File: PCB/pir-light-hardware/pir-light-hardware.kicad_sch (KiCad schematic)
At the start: 38 parts, among them J1 ZH1.5-3, J2 ZH1.5-3, Q1 AON7240, Q2 NPN, Q3 PNP, U1 M74VHC1GT08DFT2G, U2 LMV331IDCKR, U3 AS312

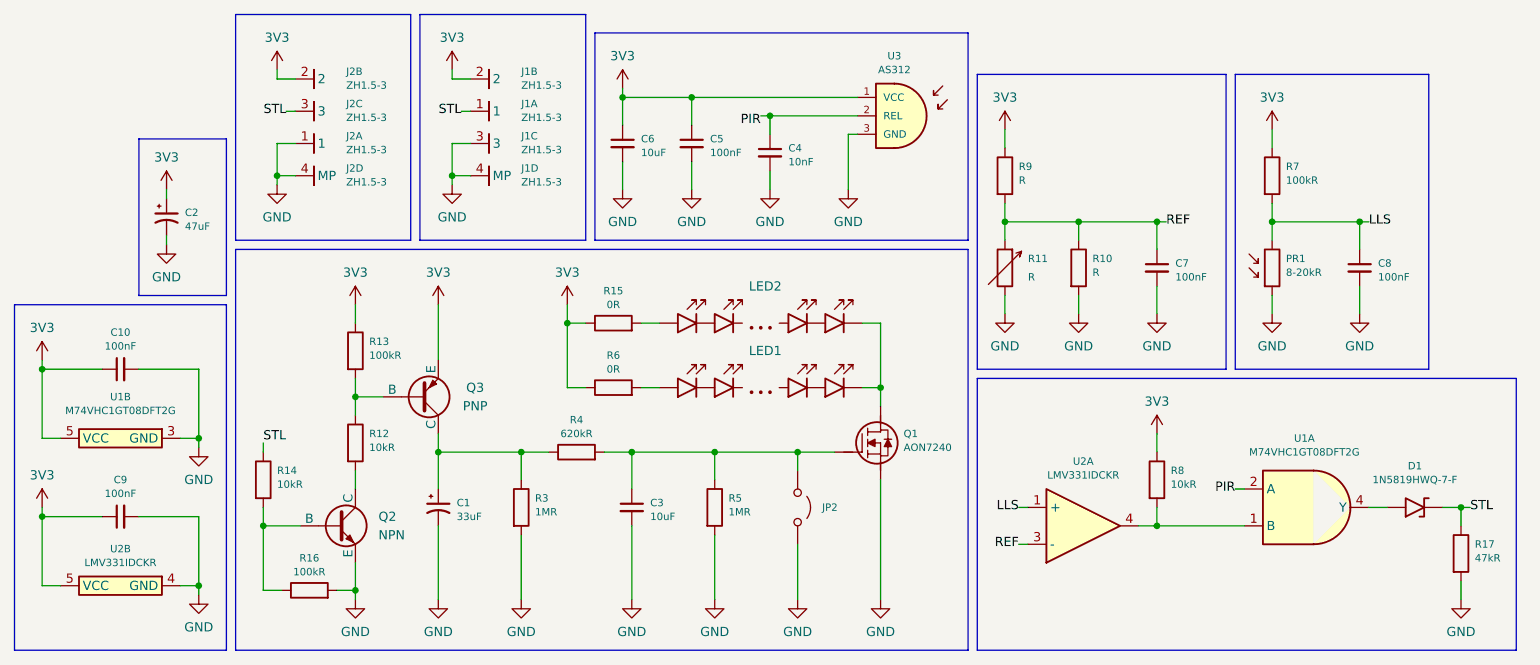
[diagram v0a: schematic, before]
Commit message: chore: add protection components
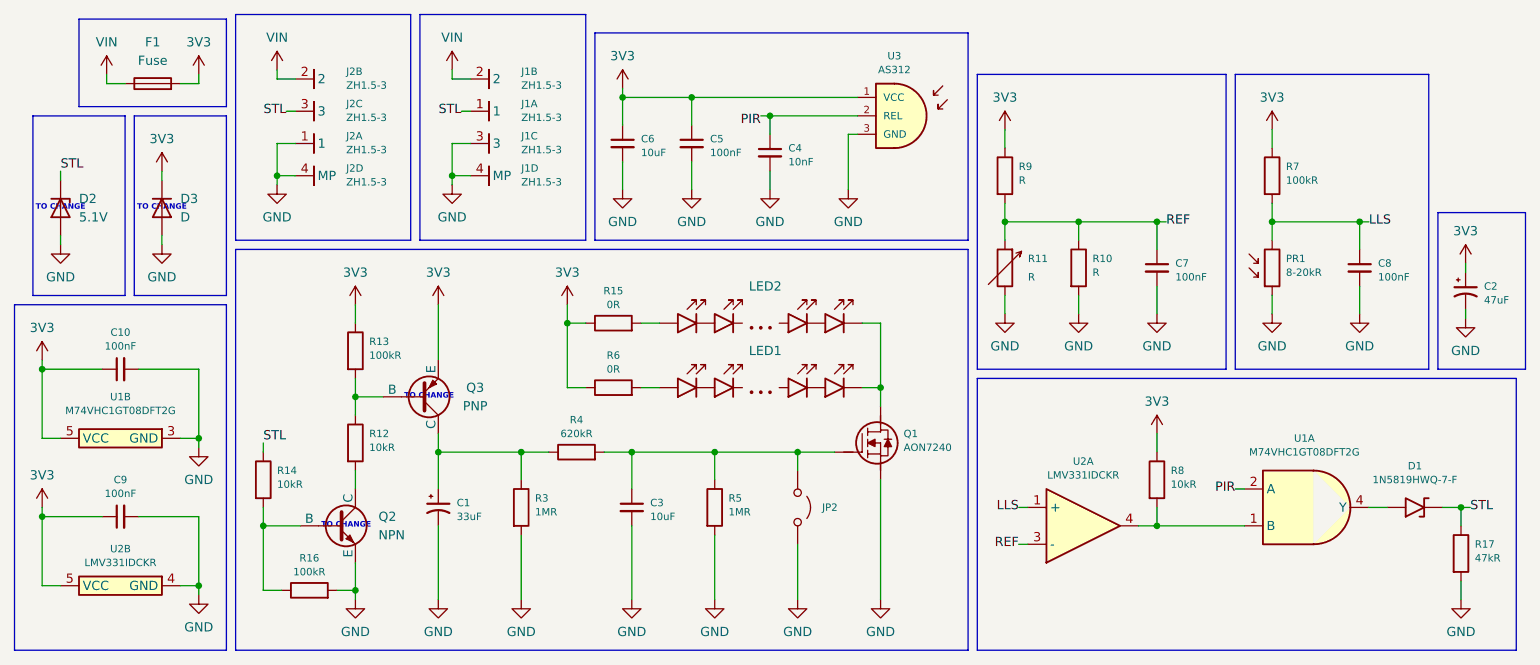
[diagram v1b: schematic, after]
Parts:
- added D2: 5.1V, symbol Device:D_Zener
- added D3: D, symbol Device:D
- added F1: Fuse, symbol Device:Fuse
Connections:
- net 3V3: now also D3.1 (K), F1.2; no longer J1.2, J2.2
- net GND: now also D2.2 (A), D3.2 (A)
- net STL: now also D2.1 (K)
- new net VIN: F1.1, J1.2, J2.2
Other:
- note added: "TO CHANGE"
- moved on the sheet: C2
